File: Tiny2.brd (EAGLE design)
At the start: 29.9 x 64.8 mm, 12 parts

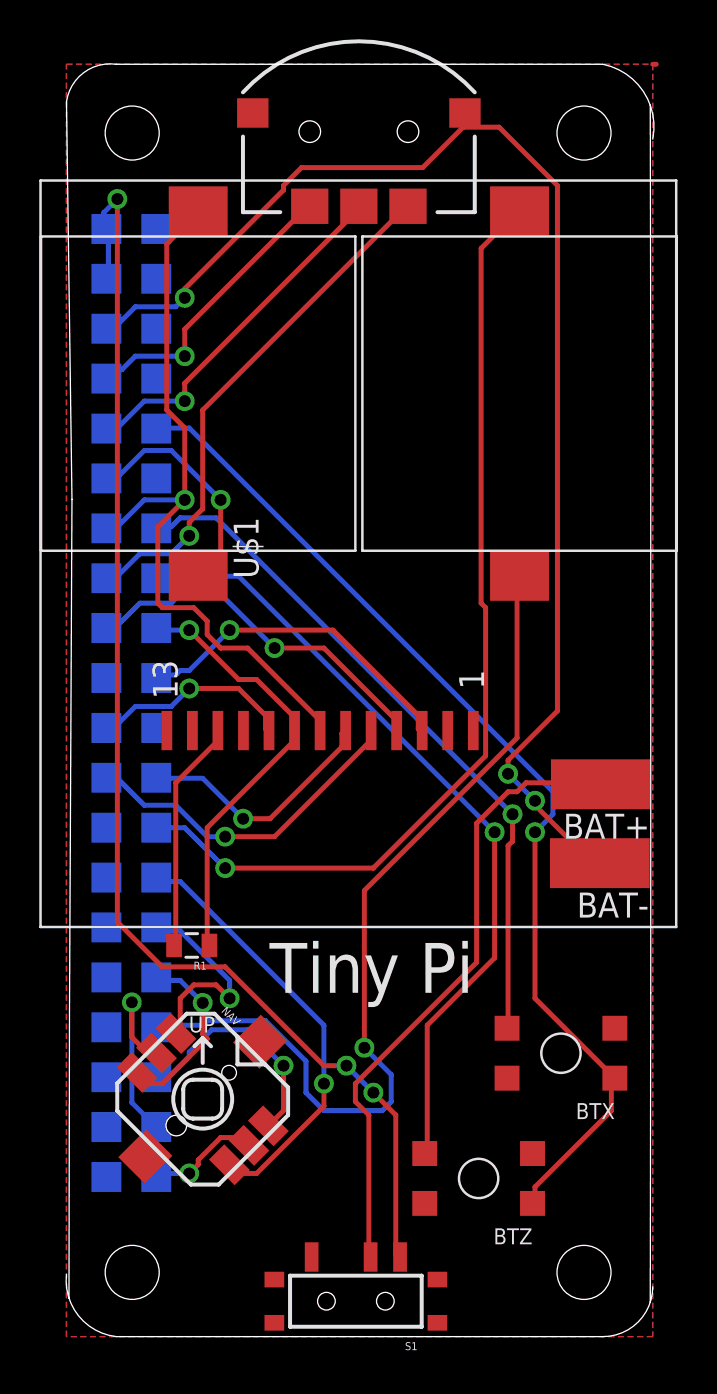
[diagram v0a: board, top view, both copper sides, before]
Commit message: Add files via upload
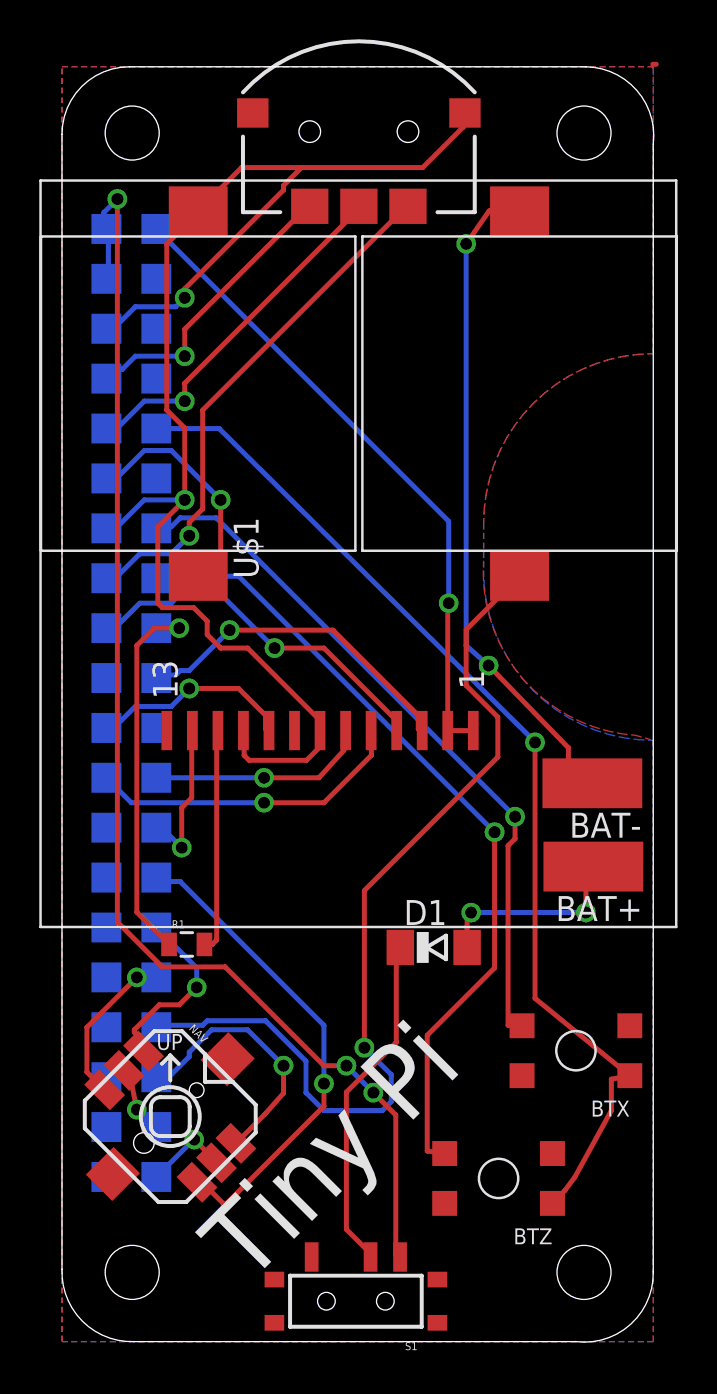
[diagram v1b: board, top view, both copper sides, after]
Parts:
- added D1: PMLL4150, diode:SOD80C
- moved BAT+ 4.21 mm to (29.7, 25.5)
- moved BAT- 4.08 mm to (29.7, 29.7)
- moved NAV 1.88 mm to (8.18, 12.7)
- moved BTZ 1.02 mm to (27.6, 8.31)
- moved BTX 0.77 mm to (31.6, 14.8)
- moved R1 0.26 mm to (9.02, 21.5), turned to 0 degrees
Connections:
- removed net GND@4: PI1.14, SG1.P$2, U$1.P$7
- removed net N$19: PI1.17, R1.1, U$1.P$8
- removed net N$24: BAT+.1, S1.P
- new net 3V3@1: PI1.1, U$1.P$1, U$1.P$2
- new net 3V3@2: PI1.17, R1.1
- new net N$20: BAT+.1, D1.A
- new net N$21: D1.C, S1.P
- net GND@2: now also U$1.P$12; no longer SG2.P$2
- net GND@8: now also SG1.P$2, SG2.P$2, U$1.P$10, U$1.P$7
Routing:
- net GND@2: track 48.6 -> 7.90 mm
- net GND@8: track 68.1 -> 108.4 mm, vias 3 -> 4
- net GND@4: track 37.8 -> 0.00 mm, vias 1 -> 0
- net 3V3@1: track 0.00 -> 33.0 mm, vias 0 -> 1
- net N$24: track 32.1 -> 0.00 mm
- net N$19: track 22.4 -> 0.00 mm, vias 1 -> 0
- net 3V3@2: track 0.00 -> 19.6 mm, vias 0 -> 1
- net N$21: track 0.00 -> 17.4 mm
- net N$20: track 0.00 -> 10.2 mm, vias 0 -> 2
- net N$4: track 10.2 -> 3.49 mm
- net N$10: track 22.4 -> 24.8 mm
- net N$15: track 45.7 -> 47.3 mm
- net GND@3: track 5.93 -> 4.37 mm
- net N$5: track 11.8 -> 13.3 mm
- net N$9: track 10.8 -> 9.24 mm
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- added copper zone on layer 16, net N$19
- added copper zone on layer 1, net N$25
- removed copper zone on layer 1, net N$22
- removed copper zone on layer 16, net N$23
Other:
- board size 29.9 x 64.8 mm -> 30.1 x 64.9 mm
- board text added: "#P0CKET"
- board text added: "i"
